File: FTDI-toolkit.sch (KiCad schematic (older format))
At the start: 83 parts, among them IC1 TLV70033DCKT, IC12 SN74LV1T125DCKR, IC13 74HC00BQ, IC15 TS5A3359, IC2 TLV70018DCKT, IC3 TS5A3359, IC7 SN74LV1T125DCKR, IC8 FT2232D, Y1 MQ-6.000-12-30/30/

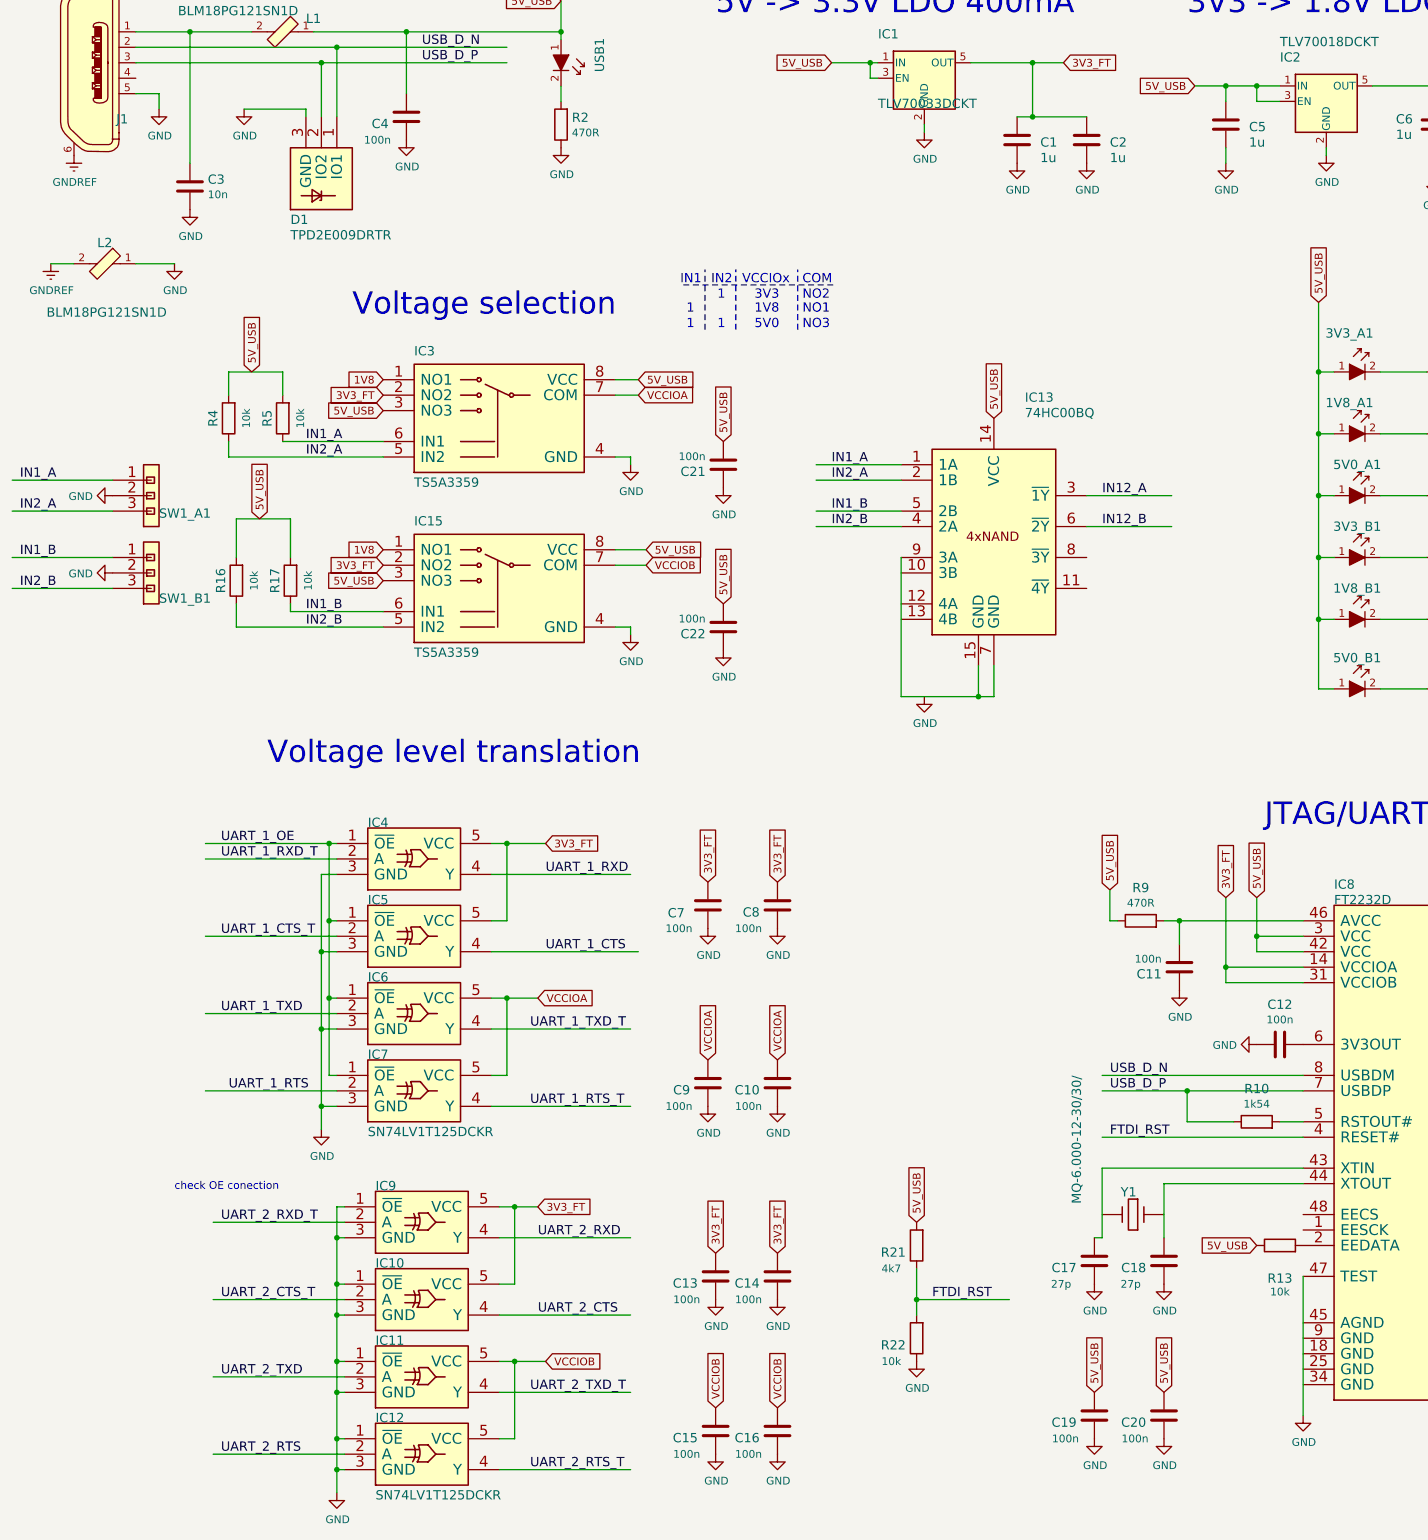
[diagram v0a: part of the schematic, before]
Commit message: Layout updates
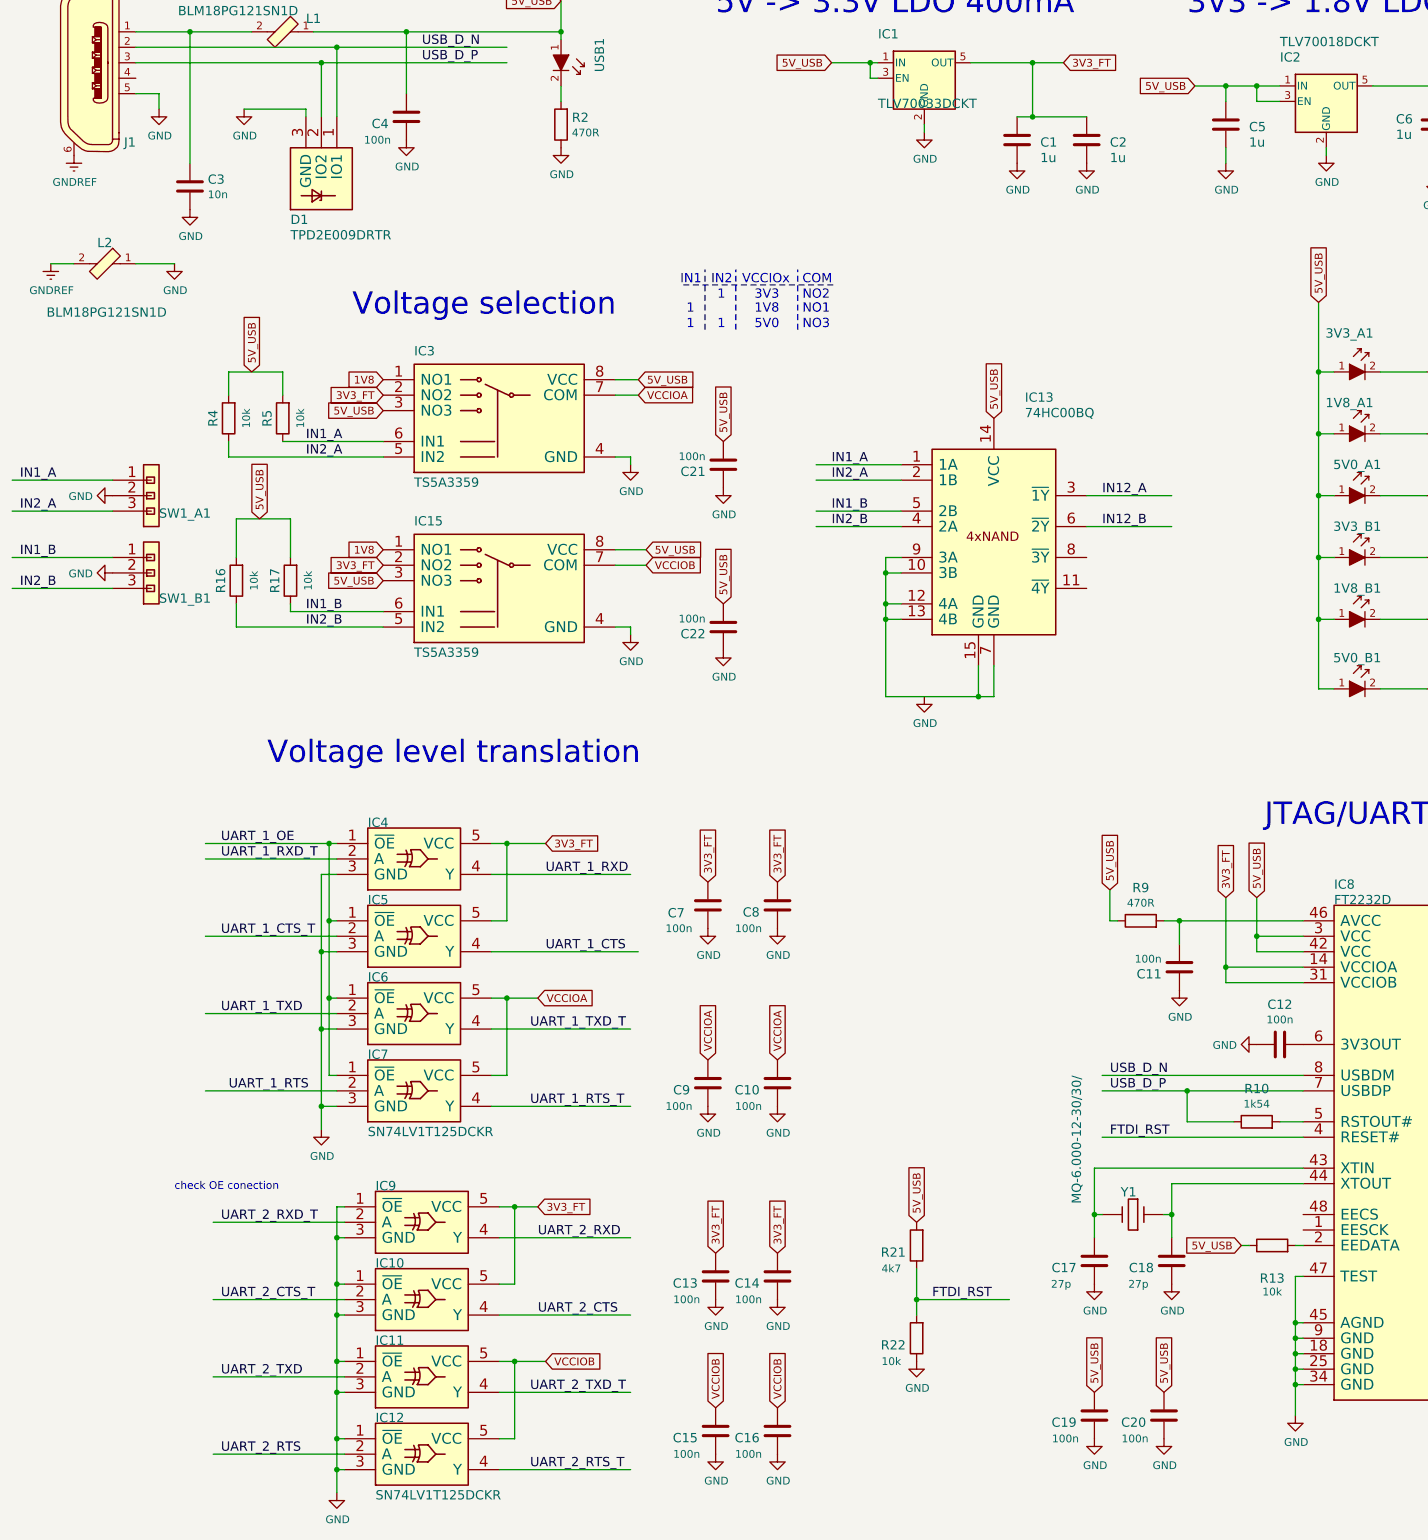
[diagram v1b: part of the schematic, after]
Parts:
- N1: footprint antmicro-footprints:antmicro-logo -> antmicro-footprints:antmicro-logo_scaled_12mm
- N2: footprint antmicro-footprints:oshw-logo -> antmicro-footprints:OSHW-Logo2_7.3x6mm_SilkScreen
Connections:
- wire segments 267 -> 290
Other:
- moved on the sheet: C18, R13
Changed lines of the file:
@@
 Wire Wire Line
 	12100 2050 12100 1800
-Wire Wire Line
-	9050 8950 8150 8950
-Wire Wire Line
-	7750 9300 7700 9300
-Text GLabel 8750 9350 0    50   Input ~ 0
+Text GLabel 8650 9350 0    50   Input ~ 0
 5V_USB
 Wire Wire Line
@@
 	3950 10100 4150 10100
 Wire Wire Line
-	7750 8850 9050 8850
+	7700 8850 9050 8850
 Text GLabel 5250 10400 1    50   Input ~ 0
 VCCIOB
@@
 Review connections!!!!
 Wire Wire Line
-	6450 5800 6950 5800
-Wire Wire Line
 	8750 1850 8750 1950
 Wire Wire Line
@@
 Wire Wire Line
 	1500 1500 1850 1500
-Wire Wire Line
-	8150 8950 8150 9300
-Wire Wire Line
-	7750 8850 7750 9300
-Wire Wire Line
-	6450 4900 6450 5800
-Wire Wire Line
-	9050 9550 9050 10450
 Wire Wire Line
 	4250 1550 4250 1500
@@
 F 0 "N2" H 11244 10853 50  0000 L CNN
 F 1 "oshw_logo" H 11244 10762 50  0000 L CNN
-F 2 "antmicro-footprints:oshw-logo" H 11070 10610 50  0001 C CNN
+F 2 "antmicro-footprints:OSHW-Logo2_7.3x6mm_SilkScreen" H 11070 10610 50  0001 C CNN
 F 3 "" H 11050 10850 50  0001 C CNN
 	1    11050 10850
@@
 F 0 "N1" H 10314 11043 50  0000 L CNN
 F 1 "antmicro_logo" H 10314 10952 50  0000 L CNN
-F 2 "antmicro-footprints:antmicro-logo" H 10000 11200 50  0001 C CNN
+F 2 "antmicro-footprints:antmicro-logo_scaled_12mm" H 10000 11200 50  0001 C CNN
 F 3 "" H 10100 11300 50  0001 C CNN
 	1    10100 10950
@@
 L antmicroResistors0402:R_10k_0402 R13
 U 1 1 5F464B54
-P 8900 9350
-F 0 "R13" H 8900 9137 60  0000 C CNN
-F 1 "R_10k_0402" H 8900 9200 60  0001 C CNN
-F 2 "antmicro-footprints:0402-res" H 9100 9550 60  0001 L CNN
-F 3 "" H 8900 9350 50  0001 C CNN
-F 4 "VISHAY" H 9100 9750 60  0001 L CNN "Manufacturer"
-F 5 "CRCW040210K0FKEDHP" H 9100 9650 60  0001 L CNN "MPN"
-F 6 "10k" H 8900 9050 50  0000 C CNN "Val"
-	1    8900 9350
+P 8850 9350
+F 0 "R13" H 8850 9137 60  0000 C CNN
+F 1 "R_10k_0402" H 8850 9200 60  0001 C CNN
+F 2 "antmicro-footprints:0402-res" H 9050 9550 60  0001 L CNN
+F 3 "" H 8850 9350 50  0001 C CNN
+F 4 "VISHAY" H 9050 9750 60  0001 L CNN "Manufacturer"
+F 5 "CRCW040210K0FKEDHP" H 9050 9650 60  0001 L CNN "MPN"
+F 6 "10k" H 8850 9050 50  0000 C CNN "Val"
+	1    8850 9350
 	1    0    0    -1
 $EndComp
@@
 L power:GND #PWR0123
 U 1 1 5FBF14DD
-P 9050 10450
-F 0 "#PWR0123" H 9050 10200 50  0001 C CNN
-F 1 "GND" H 9055 10277 50  0000 C CNN
-F 2 "" H 9050 10450 50  0001 C CNN
-F 3 "" H 9050 10450 50  0001 C CNN
-	1    9050 10450
+P 9000 10450
+F 0 "#PWR0123" H 9000 10200 50  0001 C CNN
+F 1 "GND" H 9005 10277 50  0000 C CNN
+F 2 "" H 9000 10450 50  0001 C CNN
+F 3 "" H 9000 10450 50  0001 C CNN
+	1    9000 10450
 	1    0    0    -1
 $EndComp
@@
 L power:GND #PWR0120
 U 1 1 5FB95D7E
-P 8150 9600
-F 0 "#PWR0120" H 8150 9350 50  0001 C CNN
-F 1 "GND" H 8155 9427 50  0000 C CNN
-F 2 "" H 8150 9600 50  0001 C CNN
-F 3 "" H 8150 9600 50  0001 C CNN
-	1    8150 9600
+P 8200 9600
+F 0 "#PWR0120" H 8200 9350 50  0001 C CNN
+F 1 "GND" H 8205 9427 50  0000 C CNN
+F 2 "" H 8200 9600 50  0001 C CNN
+F 3 "" H 8200 9600 50  0001 C CNN
+	1    8200 9600
 	1    0    0    -1
 $EndComp
@@
 L antmicroCapacitors0402:C_27p_0402 C18
 U 1 1 5F401E5E
-P 8150 9450
-F 0 "C18" H 8265 9495 60  0000 L CNN
-F 1 "C_27p_0402" H 8150 9300 60  0001 C CNN
-F 2 "antmicro-footprints:0402-cap" H 8350 9650 60  0001 L CNN
-F 3 "" H 8150 9450 50  0001 C CNN
-F 4 "WALSIN" H 8350 9850 60  0001 L CNN "Manufacturer"
-F 5 "0402N270J500CT" H 8350 9750 60  0001 L CNN "MPN"
-F 6 "27p" H 8300 9600 50  0000 L CNN "Val"
-	1    8150 9450
+P 8200 9450
+F 0 "C18" H 8315 9495 60  0000 L CNN
+F 1 "C_27p_0402" H 8200 9300 60  0001 C CNN
+F 2 "antmicro-footprints:0402-cap" H 8400 9650 60  0001 L CNN
+F 3 "" H 8200 9450 50  0001 C CNN
+F 4 "WALSIN" H 8400 9850 60  0001 L CNN "Manufacturer"
+F 5 "0402N270J500CT" H 8400 9750 60  0001 L CNN "MPN"
+F 6 "27p" H 8350 9600 50  0000 L CNN "Val"
+	1    8200 9450
 	-1   0    0    1
 $EndComp
@@
 U 1 1 5E5F7C20
 P 1200 1700
-F 0 "J1" H 1450 1300 60  0000 R BNN
+F 0 "J1" H 1500 1150 60  0000 R BNN
 F 1 "~" H 1200 1700 50  0001 C CNN
 F 2 "antmicro-footprints:USB_Micro_B_Female_629105150521" H 1200 1700 50  0001 C CNN
@@
 	0    1    1    0
 $EndComp
+Wire Wire Line
+	9000 9350 9050 9350
+Wire Wire Line
+	8700 9350 8650 9350
+Wire Wire Line
+	9050 9550 9000 9550
+Wire Wire Line
+	9000 9550 9000 9850
+Wire Wire Line
+	9050 10250 9000 10250
+Connection ~ 9000 10250
+Wire Wire Line
+	9000 10250 9000 10450
+Wire Wire Line
+	9050 10150 9000 10150
+Connection ~ 9000 10150
+Wire Wire Line
+	9000 10150 9000 10250
+Wire Wire Line
+	9050 10050 9000 10050
+Connection ~ 9000 10050
+Wire Wire Line
+	9000 10050 9000 10150
+Wire Wire Line
+	9050 9950 9000 9950
+Connection ~ 9000 9950
+Wire Wire Line
+	9000 9950 9000 10050
+Wire Wire Line
+	9050 9850 9000 9850
+Connection ~ 9000 9850
+Wire Wire Line
+	9000 9850 9000 9950
+Wire Wire Line
+	7700 8850 7700 9150
+Wire Wire Line
+	8200 8950 9050 8950
+Wire Wire Line
+	8200 8950 8200 9150
+Wire Wire Line
+	8150 9150 8200 9150
+Connection ~ 8200 9150
+Wire Wire Line
+	8200 9150 8200 9300
+Wire Wire Line
+	7750 9150 7700 9150
+Connection ~ 7700 9150
+Wire Wire Line
+	7700 9150 7700 9300
+Wire Wire Line
+	6450 4900 6350 4900
+Wire Wire Line
+	6350 4900 6350 5000
+Wire Wire Line
+	6350 5800 6950 5800
+Wire Wire Line
+	6450 5000 6350 5000
+Connection ~ 6350 5000
+Wire Wire Line
+	6350 5000 6350 5200
+Wire Wire Line
+	6450 5200 6350 5200
+Connection ~ 6350 5200
+Wire Wire Line
+	6350 5200 6350 5300
+Wire Wire Line
+	6450 5300 6350 5300
+Connection ~ 6350 5300
+Wire Wire Line
+	6350 5300 6350 5800
 $EndSCHEMATC
